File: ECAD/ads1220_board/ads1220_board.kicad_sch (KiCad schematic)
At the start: 34 parts, among them J2 LOAD CELL, J3 Conn_01x08, U1 TPS79301-EP, U2 INA826, U3 ADS1220xPW, U4 OPA333xxDBV

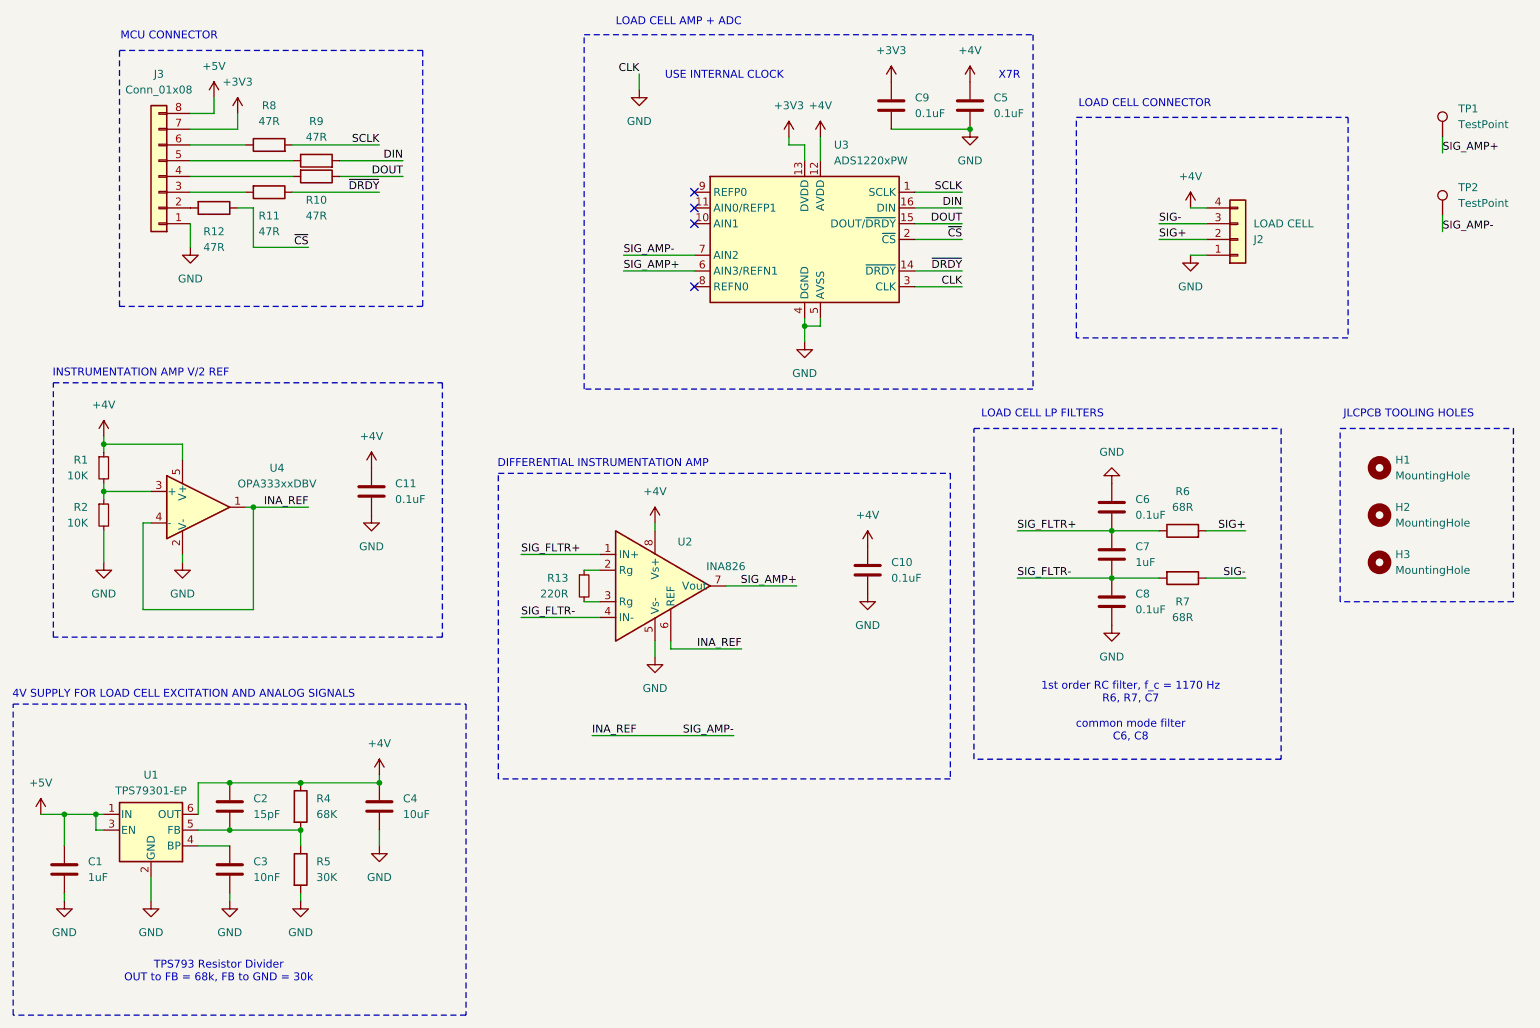
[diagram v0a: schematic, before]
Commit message: updates
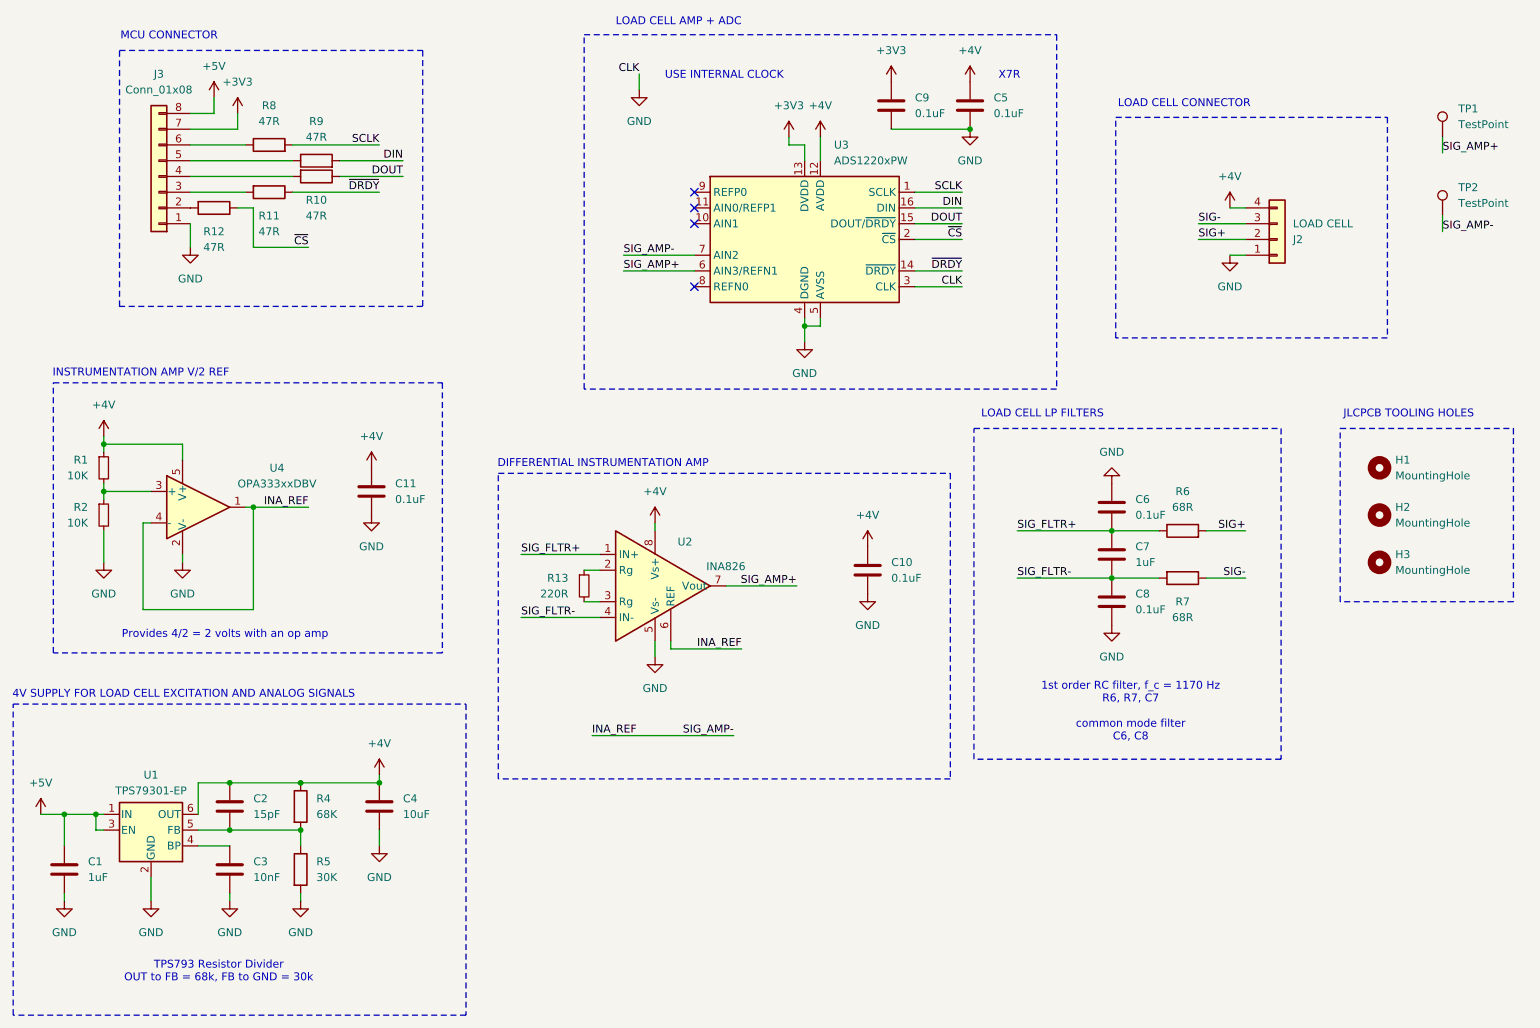
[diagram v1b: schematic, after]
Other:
- note added: "Provides 4/2 = 2 volts with an op amp"
- moved on the sheet: J2
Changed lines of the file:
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@@
 	(wire
 		(pts
-			(xy 200.66 67.31) (xy 208.28 67.31)
+			(xy 207.01 67.31) (xy 214.63 67.31)
 		)
 		(stroke
@@
 	(wire
 		(pts
-			(xy 205.74 69.85) (xy 208.28 69.85)
+			(xy 212.09 69.85) (xy 214.63 69.85)
 		)
 		(stroke
@@
 	(wire
 		(pts
-			(xy 205.74 62.23) (xy 208.28 62.23)
+			(xy 212.09 62.23) (xy 214.63 62.23)
 		)
 		(stroke
@@
 	(wire
 		(pts
-			(xy 161.29 72.39) (xy 168.91 72.39)
-		)
-		(stroke
-			(width 0)
-			(type default)
-		)
-	)
-	(wire
-		(pts
 			(xy 161.29 59.69) (xy 168.91 59.69)
 		)
@@
 	(wire
 		(pts
-			(xy 200.66 64.77) (xy 208.28 64.77)
+			(xy 207.01 64.77) (xy 214.63 64.77)
 		)
 		(stroke
@@
 	(wire
 		(pts
+			(xy 161.29 72.39) (xy 168.91 72.39)
+		)
+		(stroke
+			(width 0)
+			(type default)
+		)
+	)
+	(wire
+		(pts
 			(xy 143.51 52.07) (xy 143.51 54.61)
 		)
@@
 	)
 	(rectangle
-		(start 187.325 47.625)
-		(end 231.14 83.185)
+		(start 193.675 47.625)
+		(end 237.49 83.185)
 		(stroke
 			(width 0)
@@
 	(rectangle
 		(start 107.95 34.29)
-		(end 180.34 91.44)
+		(end 184.15 91.44)
 		(stroke
 			(width 0)
@@
 	(rectangle
 		(start 22.352 90.424)
-		(end 85.09 131.445)
+		(end 85.09 133.985)
 		(stroke
 			(width 0)
@@
 		)
 	)
+	(text "Provides 4/2 = 2 volts with an op amp"
+		(exclude_from_sim no)
+		(at 50.038 131.064 0)
+		(effects
+			(font
+				(size 1.27 1.27)
+			)
+		)
+	)
 	(text "JLCPCB TOOLING HOLES"
 		(exclude_from_sim no)
@@
 	(text "LOAD CELL CONNECTOR"
 		(exclude_from_sim no)
-		(at 198.374 45.466 0)
+		(at 204.724 45.466 0)
 		(effects
 			(font
@@
 	)
 	(label "SIG+"
-		(at 200.66 67.31 0)
+		(at 207.01 67.31 0)
 		(fields_autoplaced yes)
 		(effects
@@
 	)
 	(label "SIG-"
-		(at 200.66 64.77 0)
+		(at 207.01 64.77 0)
 		(fields_autoplaced yes)
 		(effects
@@
 	(symbol
 		(lib_id "power:+4V")
-		(at 205.74 62.23 0)
+		(at 212.09 62.23 0)
 		(unit 1)
 		(exclude_from_sim no)
@@
 		(fields_autoplaced yes)
 		(property "Reference" "#PWR020"
-			(at 205.74 66.04 0)
+			(at 212.09 66.04 0)
 			(effects
 				(font
@@
 		)
 		(property "Value" "+4V"
-			(at 205.74 57.15 0)
+			(at 212.09 57.15 0)
 			(effects
 				(font
@@
 		)
 		(property "Footprint" ""
-			(at 205.74 62.23 0)
+			(at 212.09 62.23 0)
 			(effects
 				(font
@@
 		)
 		(property "Datasheet" ""
-			(at 205.74 62.23 0)
+			(at 212.09 62.23 0)
 			(effects
 				(font
@@
 		)
 		(property "Description" "Power symbol creates a global label with name \"+4V\""
-			(at 205.74 62.23 0)
+			(at 212.09 62.23 0)
 			(effects
 				(font
@@
 	(symbol
 		(lib_id "power:GND")
-		(at 205.74 69.85 0)
+		(at 212.09 69.85 0)
 		(unit 1)
 		(exclude_from_sim no)
@@
 		(fields_autoplaced yes)
 		(property "Reference" "#PWR021"
-			(at 205.74 76.2 0)
+			(at 212.09 76.2 0)
 			(effects
 				(font
@@
 		)
 		(property "Value" "GND"
-			(at 205.74 74.93 0)
+			(at 212.09 74.93 0)
 			(effects
 				(font
@@
 		)
 		(property "Footprint" ""
-			(at 205.74 69.85 0)
+			(at 212.09 69.85 0)
 			(effects
 				(font
@@
 		)
 		(property "Datasheet" ""
-			(at 205.74 69.85 0)
+			(at 212.09 69.85 0)
 			(effects
 				(font
@@
 		)
 		(property "Description" "Power symbol creates a global label with name \"GND\" , ground"
-			(at 205.74 69.85 0)
+			(at 212.09 69.85 0)
 			(effects
 				(font
@@
 	(symbol
 		(lib_id "Connector_Generic:Conn_01x04")
-		(at 213.36 67.31 0)
+		(at 219.71 67.31 0)
 		(mirror x)
 		(unit 1)
@@
 		(dnp no)
 		(property "Reference" "J2"
-			(at 215.9 67.3101 0)
+			(at 222.25 67.3101 0)
 			(effects
 				(font
@@
 		)
 		(property "Value" "LOAD CELL"
-			(at 215.9 64.7701 0)
+			(at 222.25 64.7701 0)
 			(effects
 				(font
@@
 		)
 		(property "Footprint" "Connector_JST:JST_PH_B4B-PH-K_1x04_P2.00mm_Vertical"
-			(at 213.36 67.31 0)
+			(at 219.71 67.31 0)
 			(effects
 				(font
@@
 		)
 		(property "Datasheet" "~"
-			(at 213.36 67.31 0)
+			(at 219.71 67.31 0)
 			(effects
 				(font
@@
 		)
 		(property "Description" "Generic connector, single row, 01x04, script generated (kicad-library-utils/schlib/autogen/connector/)"
-			(at 213.36 67.31 0)
+			(at 219.71 67.31 0)
 			(effects
 				(font
@@
 		)
 		(property "JLC PN" ""
-			(at 213.36 67.31 0)
+			(at 219.71 67.31 0)
 			(effects
 				(font
